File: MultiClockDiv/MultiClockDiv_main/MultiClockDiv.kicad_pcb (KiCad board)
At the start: 2 copper layers, 38.1 x 105 mm, 32 parts, among them J1 GATE OUT1, J2 GATE OUT2, J3 MASTER CLOCK OUT, J4 EXTERNAL CLOCK IN, J5 Conn_01x16_Male, SW1 SW_SPDT

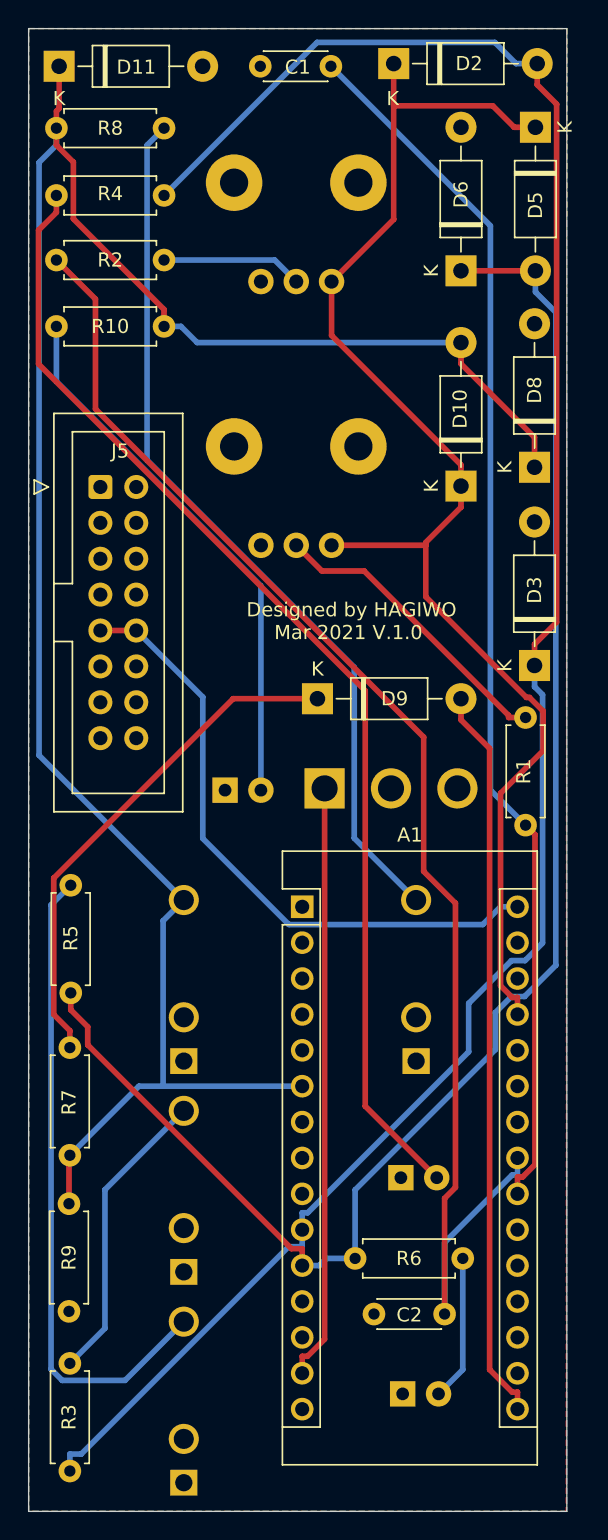
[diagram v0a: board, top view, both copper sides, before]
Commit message: First commit
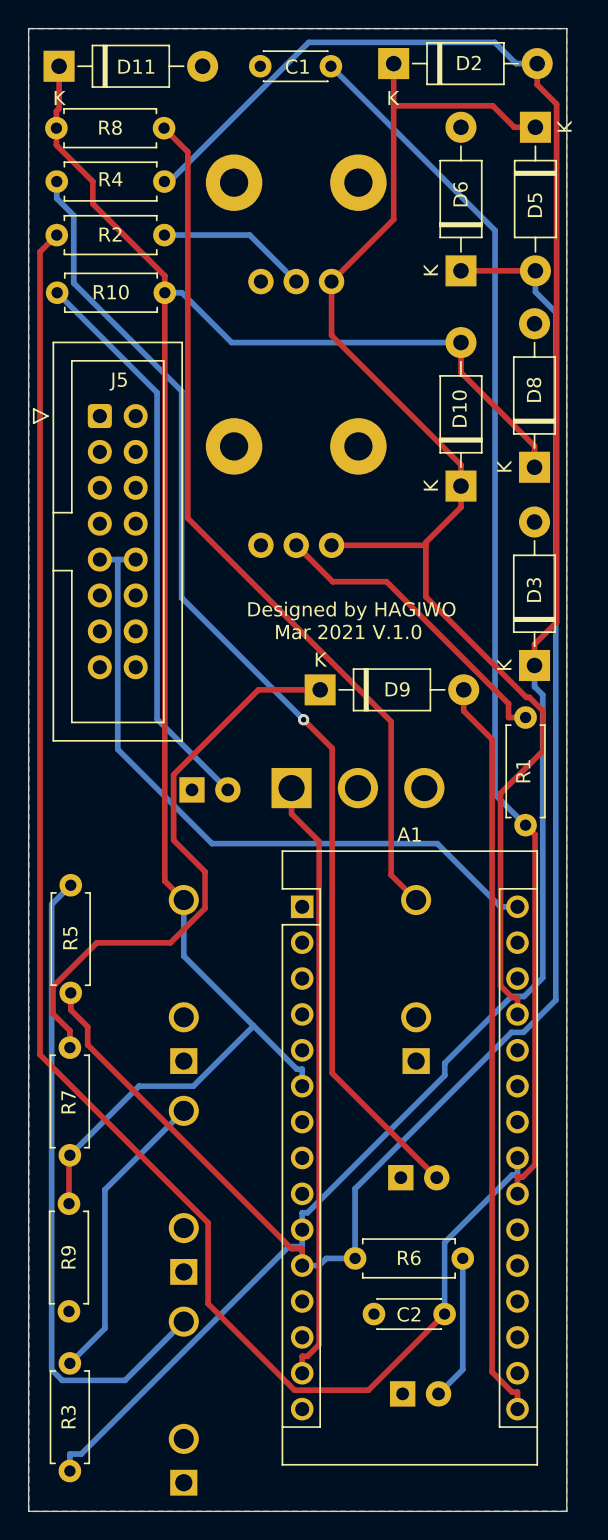
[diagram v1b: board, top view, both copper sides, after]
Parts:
- moved J5 5.02 mm to (166.8, 75.2)
- moved R10 2.38 mm to (163.8, 66.5)
- moved D7 2.34 mm to (173.4, 101.6)
- moved SW1 2.34 mm to (180.4, 101.5)
- moved R2 1.77 mm to (163.8, 62.4)
- moved R4 0.98 mm to (171.4, 58.6)
- moved D9 0.66 mm to (182.4, 94.6)
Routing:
- net Net-(A1-Pad23): track 100.0 -> 116.0 mm
- net Net-(A1-Pad6): track 149.2 -> 133.4 mm
- net Net-(D9-Pad1): track 36.4 -> 41.1 mm
- net 12V: track 44.5 -> 48.9 mm
- net Net-(D7-Pad2): track 38.8 -> 40.2 mm
- net Net-(J4-PadT): track 63.0 -> 62.0 mm
- net Net-(R2-Pad2): track 9.99 -> 10.7 mm
- net Net-(A1-Pad14): track 42.3 -> 42.9 mm
- net Net-(A1-Pad16): track 52.2 -> 52.7 mm
- net Net-(D1-Pad2): vias 0 -> 1
